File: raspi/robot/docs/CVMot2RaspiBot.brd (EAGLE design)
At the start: 64 x 58 mm, 2 parts

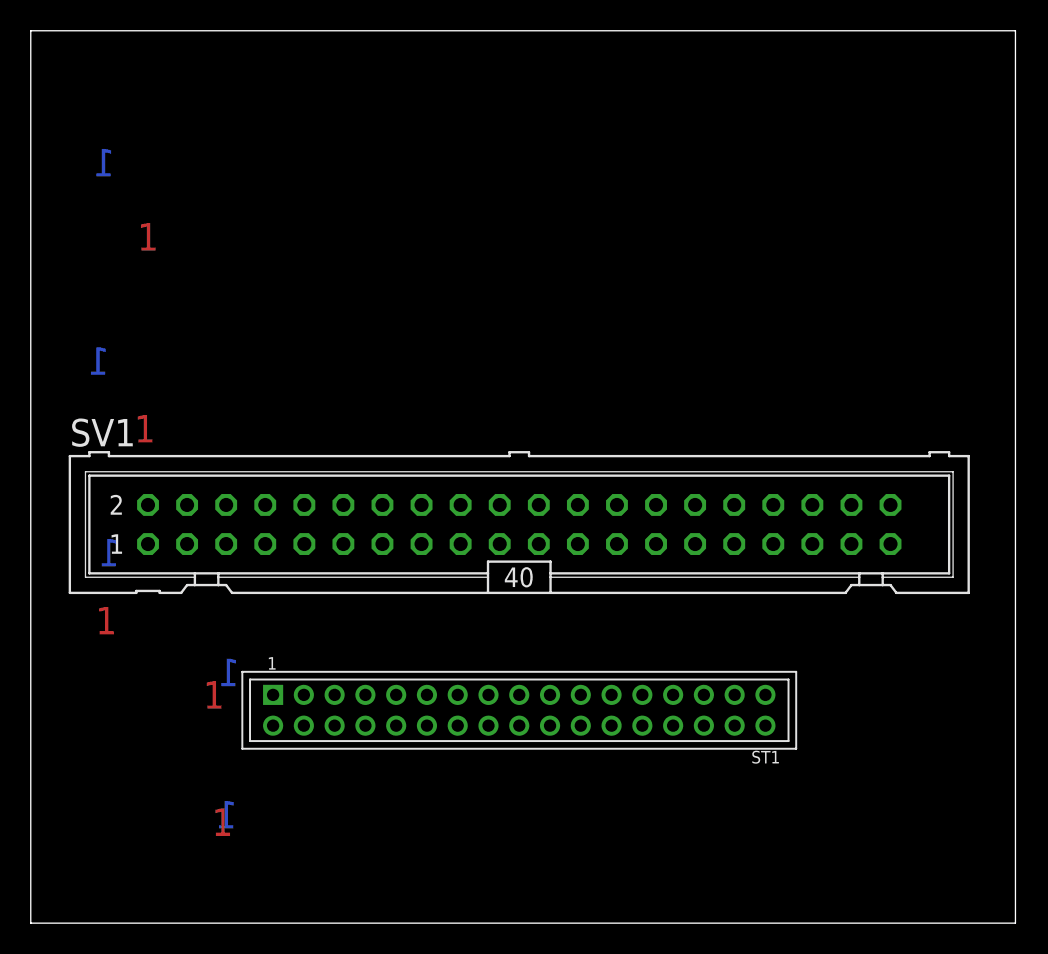
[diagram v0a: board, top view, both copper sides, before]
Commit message: Raspi: Update Schaltpläne
git-svn-id: https://cvsvn/svn/raspi/trunk@93 50237d99-7d21-444e-87dd-016511c29f8c
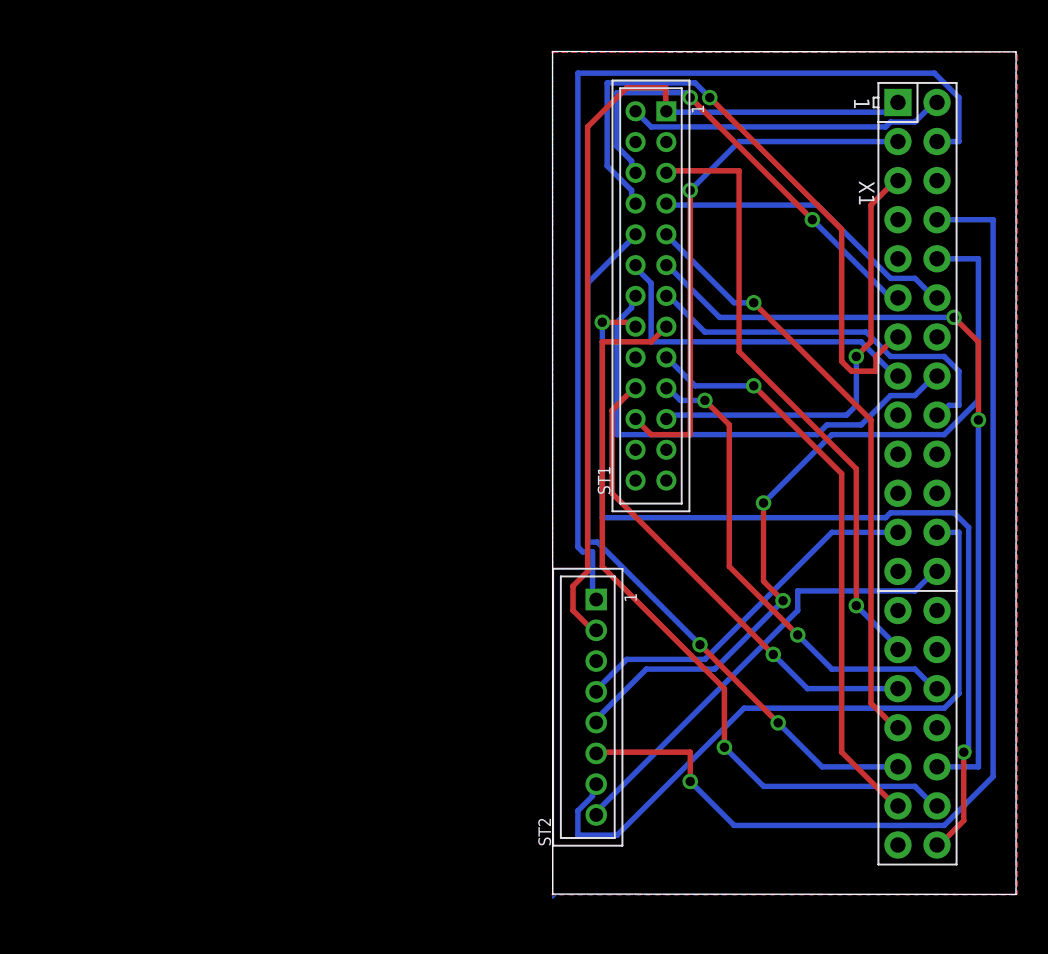
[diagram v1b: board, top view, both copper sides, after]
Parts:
- removed SV1: (no value), con-harting-ml:ML40
- added ST2: B8B-PH-K-S, CV_Con:JST-PH_8_TH
- added X1: RASPI_GPIO_B+#_PIN, raspberrypi_bastelstube_v13:RASPI_GPIO_B+_PIN
- ST1: value (none) -> B26B-PHDSS; device CV_Con:JST-PHD_34_TH -> CV_Con:JST-PHD_26_TH
- moved ST1 28.3 mm to (40.3, 40.8), turned to 90 degrees
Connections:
- new net 3V3B: X1.17
- new net GND: ST1.25, ST1.26, ST1.3, ST1.4, ST2.3, X1.14, X1.20, X1.25, X1.30, X1.34, X1.39, X1.6, X1.9
- new net M1_CURRENT: ST1.6, X1.11
- new net M1_DIR: ST1.8, X1.13
- new net M1_STEP: ST1.7, X1.12
- new net MOTOR_RESET: ST1.5, X1.29
- new net N$10: ST1.19, X1.32
- new net N$11: ST1.20, X1.31
- new net N$19: ST2.4, X1.23
- new net N$20: ST1.2, X1.2
- new net N$21: ST1.1, ST2.2, X1.1
- new net N$22: ST1.21, X1.5
- new net N$23: ST1.22, X1.3
- new net N$24: ST2.1, X1.4
- new net N$27: ST2.5, X1.10
- new net N$28: ST2.6, X1.8
- new net N$29: ST2.7, X1.24
- new net N$30: ST2.8, X1.26
- new net N$6: ST1.13, X1.18
- new net N$7: ST1.15, X1.38
- new net N$8: ST1.17, X1.37
- new net N$9: ST1.16, X1.40
- net N$1: now also ST1.9, X1.33; no longer ST1.5, SV1.5
- net N$2: now also ST1.11, X1.36; no longer ST1.6, SV1.3
- net N$3: now also ST1.10, X1.35; no longer ST1.8, SV1.7
- net N$4: now also ST1.12, X1.15; no longer ST1.7, SV1.8
- net N$5: now also ST1.14, X1.16; no longer ST1.3, SV1.6
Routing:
- net N$28: track 0.00 -> 70.1 mm, vias 0 -> 1
- net N$24: track 0.00 -> 64.8 mm
- net N$9: track 0.00 -> 61.1 mm, vias 0 -> 2
- net N$21: track 0.00 -> 56.8 mm
- net N$2: track 0.00 -> 52.6 mm, vias 0 -> 2
- net N$27: track 0.00 -> 51.0 mm, vias 0 -> 2
- net N$7: track 0.00 -> 49.6 mm, vias 0 -> 1
- net N$3: track 0.00 -> 47.5 mm, vias 0 -> 2
- net N$29: track 0.00 -> 44.3 mm
- net M1_DIR: track 0.00 -> 41.8 mm, vias 0 -> 1
- net MOTOR_RESET: track 0.00 -> 40.4 mm, vias 0 -> 1
- net N$1: track 0.00 -> 39.1 mm, vias 0 -> 1
- net N$8: track 0.00 -> 37.7 mm, vias 0 -> 1
- net N$23: track 0.00 -> 34.7 mm, vias 0 -> 1
- net N$5: track 0.00 -> 32.0 mm
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- added copper zone on layer 1, net GND
- added copper zone on layer 16, net GND
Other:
- board size 64 x 58 mm -> 30.1 x 54.8 mm
- board text removed: "1"
